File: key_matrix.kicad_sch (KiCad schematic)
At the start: 97 parts

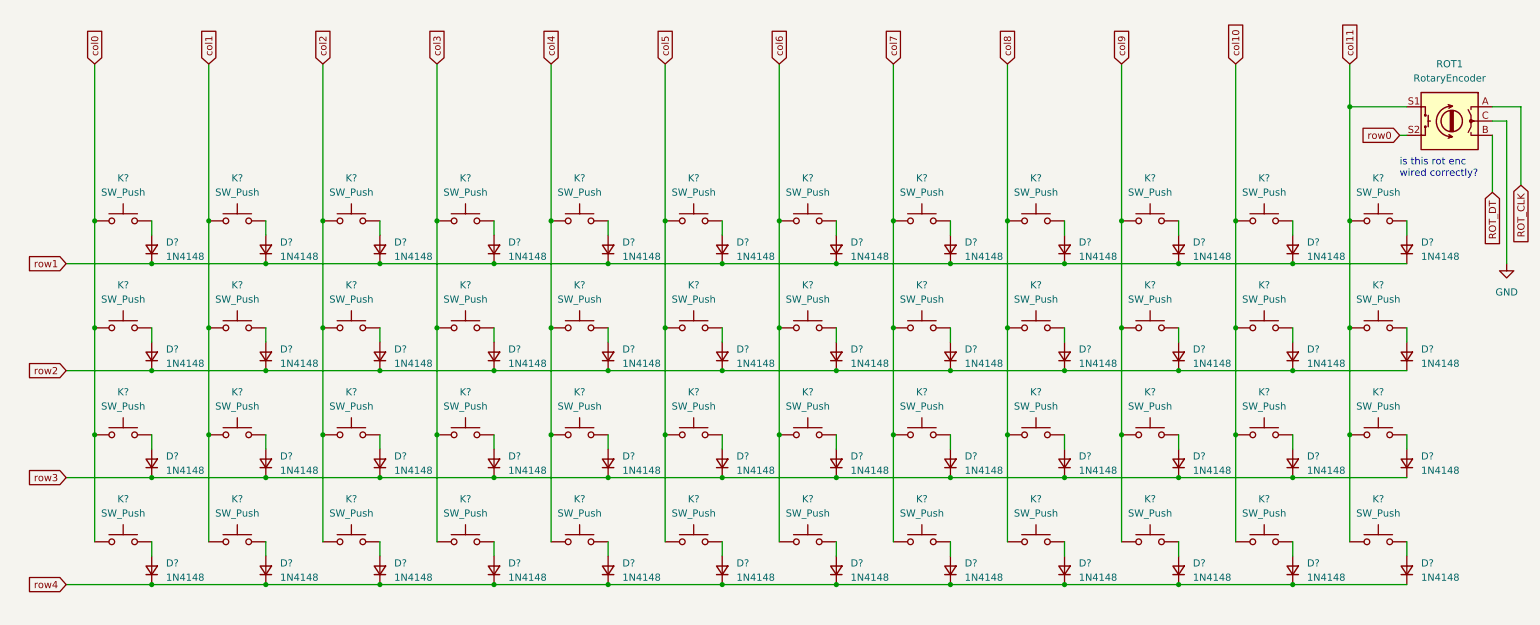
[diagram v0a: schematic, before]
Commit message: complete main circuitry
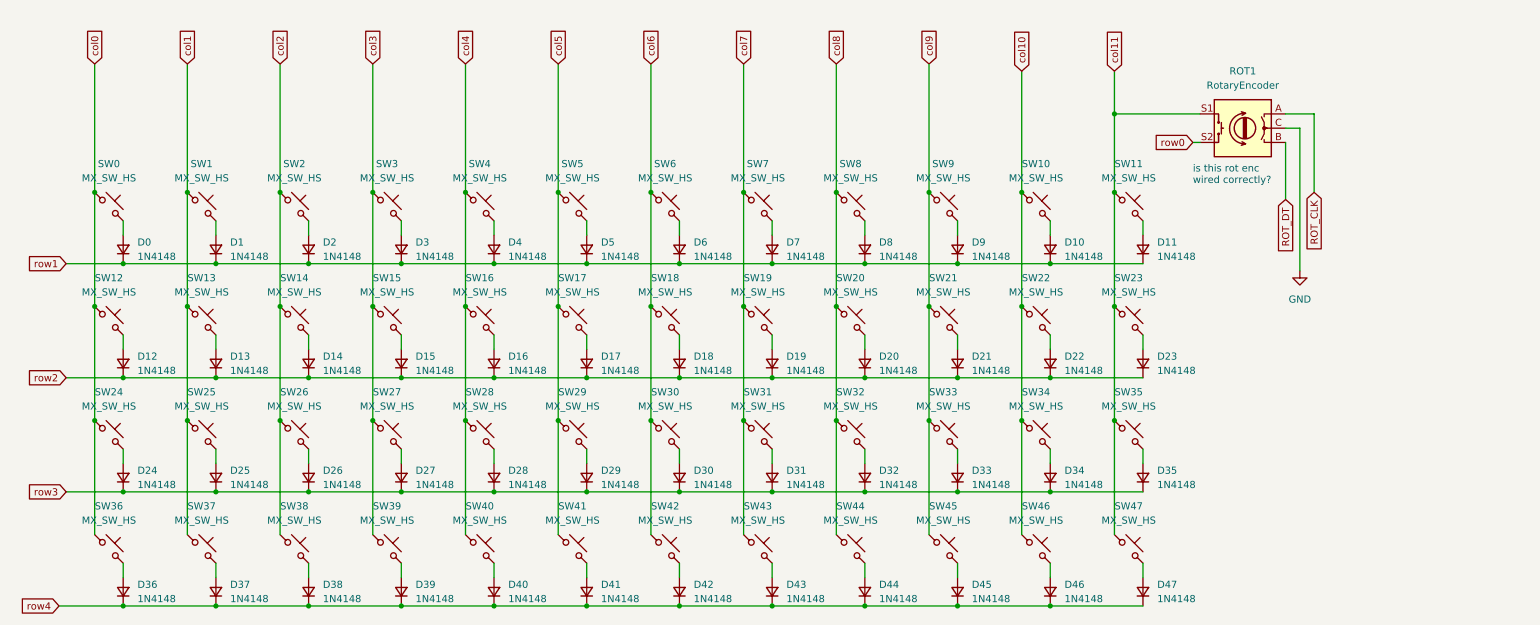
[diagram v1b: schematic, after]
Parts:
- removed D? (x47): 1N4148, symbol Device:D_Small
- removed K? (x48): SW_Push, symbol Switch:SW_Push
- added D1, D10, D11, D12, D13, D14, D15, D16, D17, D18, D19, D2, D20, D21, D22, D23, D24, D25, D26, D27, D28, D29, D3, D30, D31, D32, D33, D34, D35, D36, D37, D38, D39, D4, D40, D41, D42, D43, D44, D45, D46, D47, D5, D6, D7, D8, D9: 1N4148, symbol Device:D_Small
- added SW0, SW1, SW10, SW11, SW12, SW13, SW14, SW15, SW16, SW17, SW18, SW19, SW2, SW20, SW21, SW22, SW23, SW24, SW25, SW26, SW27, SW28, SW29, SW3, SW30, SW31, SW32, SW33, SW34, SW35, SW36, SW37, SW38, SW39, SW4, SW40, SW41, SW42, SW43, SW44, SW45, SW46, SW47, SW5, SW6, SW7, SW8, SW9: MX_SW_HS, marbastlib-mx:SW_MX_HS_1u, symbol marbastlib-mx:MX_SW_HS
- gave numbers to parts that had none: 1
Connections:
- net col0: now also SW0.1, SW12.1, SW24.1, SW36.1
- net col1: now also SW1.1, SW13.1, SW25.1, SW37.1
- net col10: now also SW10.1, SW22.1, SW34.1, SW46.1
- net col11: now also SW11.1, SW23.1, SW35.1, SW47.1
- net col2: now also SW14.1, SW2.1, SW26.1, SW38.1
- net col3: now also SW15.1, SW27.1, SW3.1, SW39.1
- net col4: now also SW16.1, SW28.1, SW4.1, SW40.1
- net col5: now also SW17.1, SW29.1, SW41.1, SW5.1
- net col6: now also SW18.1, SW30.1, SW42.1, SW6.1
- net col7: now also SW19.1, SW31.1, SW43.1, SW7.1
- net col8: now also SW20.1, SW32.1, SW44.1, SW8.1
- net col9: now also SW21.1, SW33.1, SW45.1, SW9.1
- net row1: now also D1.1 (K), D10.1 (K), D11.1 (K), D2.1 (K), D3.1 (K), D4.1 (K), D5.1 (K), D6.1 (K), D7.1 (K), D8.1 (K), D9.1 (K)
- net row2: now also D12.1 (K), D13.1 (K), D14.1 (K), D15.1 (K), D16.1 (K), D17.1 (K), D18.1 (K), D19.1 (K), D20.1 (K), D21.1 (K), D22.1 (K), D23.1 (K)
- net row3: now also D24.1 (K), D25.1 (K), D26.1 (K), D27.1 (K), D28.1 (K), D29.1 (K), D30.1 (K), D31.1 (K), D32.1 (K), D33.1 (K), D34.1 (K), D35.1 (K)
- net row4: now also D36.1 (K), D37.1 (K), D38.1 (K), D39.1 (K), D40.1 (K), D41.1 (K), D42.1 (K), D43.1 (K), D44.1 (K), D45.1 (K), D46.1 (K), D47.1 (K)
- net at D0.2 (A): now also SW0.2
- new net: D35.2 (A), SW35.2
- new net: D32.2 (A), SW32.2
- new net: D24.2 (A), SW24.2
- new net: D28.2 (A), SW28.2
- new net: D45.2 (A), SW45.2
- new net: D44.2 (A), SW44.2
- new net: D3.2 (A), SW3.2
- new net: D16.2 (A), SW16.2
- new net: D21.2 (A), SW21.2
- new net: D37.2 (A), SW37.2
- new net: D46.2 (A), SW46.2
- new net: D26.2 (A), SW26.2
- new net: D8.2 (A), SW8.2
- new net: D27.2 (A), SW27.2
- new net: D1.2 (A), SW1.2
- new net: D42.2 (A), SW42.2
- new net: D2.2 (A), SW2.2
- new net: D18.2 (A), SW18.2
- new net: D22.2 (A), SW22.2
- new net: D14.2 (A), SW14.2
- new net: D31.2 (A), SW31.2
- new net: D38.2 (A), SW38.2
- new net: D29.2 (A), SW29.2
- new net: D11.2 (A), SW11.2
- new net: D10.2 (A), SW10.2
- new net: D6.2 (A), SW6.2
- new net: D19.2 (A), SW19.2
- new net: D40.2 (A), SW40.2
- new net: D33.2 (A), SW33.2
- new net: D17.2 (A), SW17.2
- new net: D4.2 (A), SW4.2
- new net: D25.2 (A), SW25.2
- new net: D47.2 (A), SW47.2
- new net: D34.2 (A), SW34.2
- new net: D15.2 (A), SW15.2
- new net: D12.2 (A), SW12.2
- new net: D13.2 (A), SW13.2
- new net: D9.2 (A), SW9.2
- new net: D7.2 (A), SW7.2
- new net: D43.2 (A), SW43.2
- new net: D39.2 (A), SW39.2
- new net: D23.2 (A), SW23.2
- new net: D36.2 (A), SW36.2
- new net: D20.2 (A), SW20.2
- new net: D41.2 (A), SW41.2
- new net: D5.2 (A), SW5.2
- new net: D30.2 (A), SW30.2
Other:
- moved on the sheet: D0, ROT1
